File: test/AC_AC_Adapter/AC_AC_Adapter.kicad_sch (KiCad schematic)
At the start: 22 parts, among them Q1 MJE13003, Q2 BC547

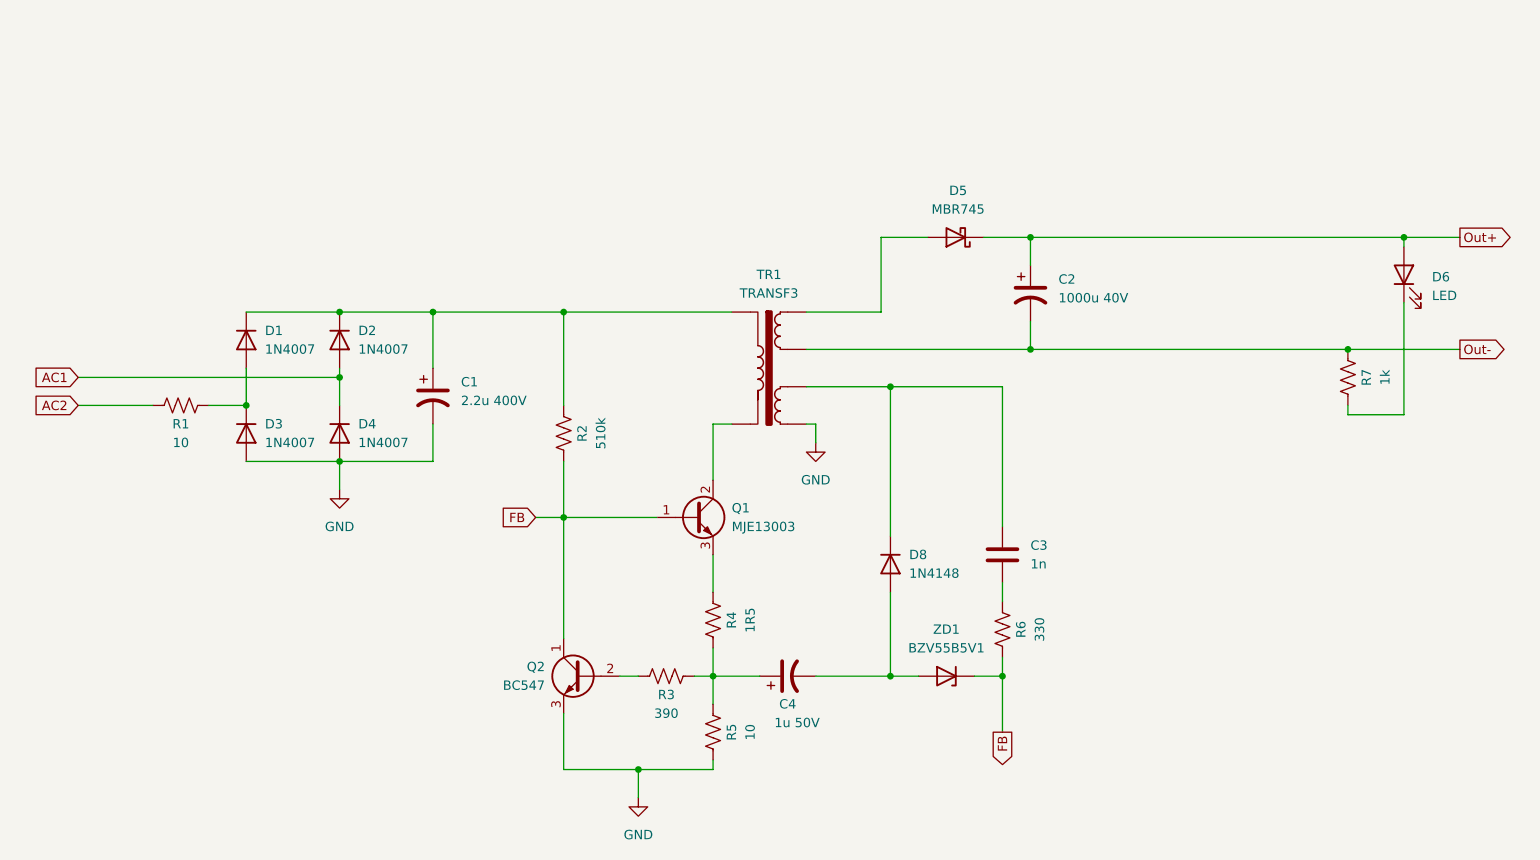
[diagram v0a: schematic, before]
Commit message: test schematic update
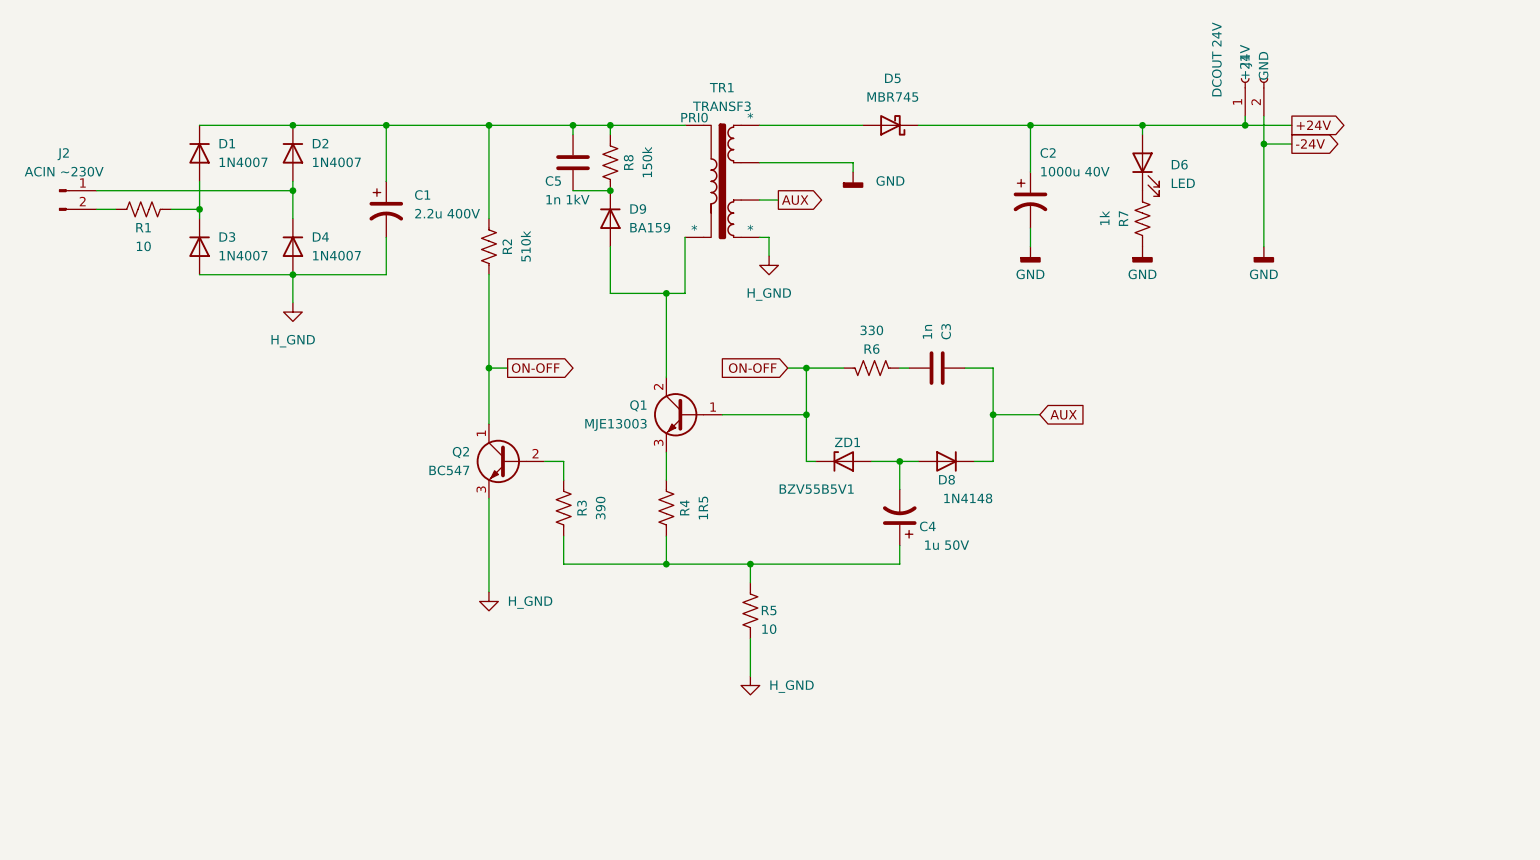
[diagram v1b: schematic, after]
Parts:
- added C5: 1n 1kV, symbol Device:C
- added D9: BA159, Diode_THT:D_DO-41_SOD81_P10.16mm_Horizontal, symbol Diode:BA159
- added J1: DCOUT 24V, symbol Connector:Conn_01x02_Socket
- added J2: ACIN ~230V, symbol Connector:Conn_01x02_Pin
- added R8: 150k, symbol Device:R_US
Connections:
- net Out- is gone; now on net GND: C2.2, R7.2, TR1.4
- net GND: now also J1.2 (GND); no longer C1.2, D3.2 (A), D4.2 (A), Q2.3 (E), R5.1, TR1.6
- net at Q2.2 (B): now also R3.2; no longer R3.1
- net at C4.1, R4.1, R5.2: now also R3.1; no longer R3.2
- net AUX: now reaches C3.1, D8.1 (K), TR1.5
- net at C1.1, D1.1 (K), D2.1 (K)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: now also C5.1, R8.2
- net at Q1.2 (C), TR1.2 (*): now also D9.2 (A)
- net AC1: no longer names the net of D2.2 (A), D4.1 (K)
- net AC1: now also J2.1 (Pin_1)
- net AC2: no longer names the net of R1.1
- net AC2: now also J2.2 (Pin_2)
- net FB renamed ON-OFF
- net Out+ renamed +24V
- net +24V: now also J1.1 (+24V)
- new net: C5.2, D9.1 (K), R8.1
- new net H_GND: C1.2, D3.2 (A), D4.2 (A), Q2.3 (E), R5.1, TR1.6 (*)
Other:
- moved on the sheet: C1, C2, C3, C4, D1, D2, D3, D4, D5, D6, D8, Q1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
